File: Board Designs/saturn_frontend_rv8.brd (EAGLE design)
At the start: 38.5 x 30.2 mm, 24 parts

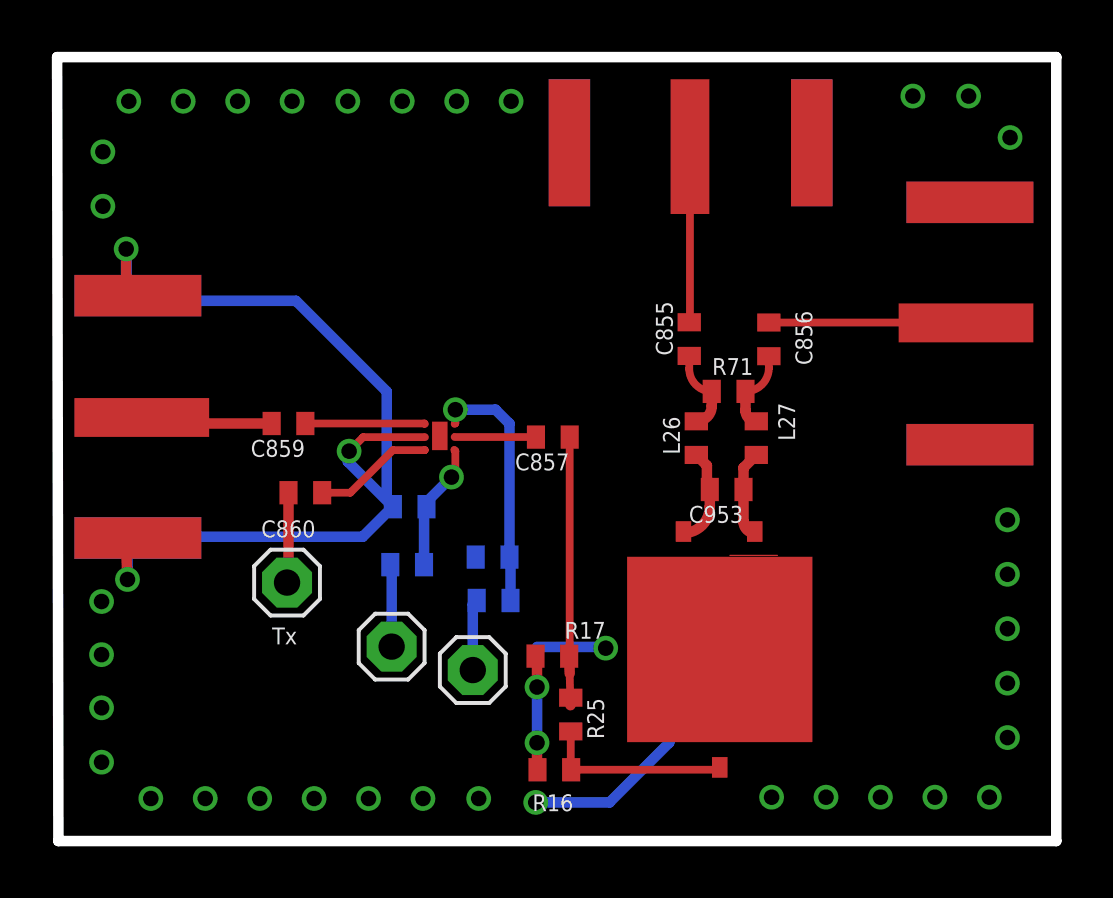
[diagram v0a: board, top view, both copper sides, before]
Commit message: Next Revision of board
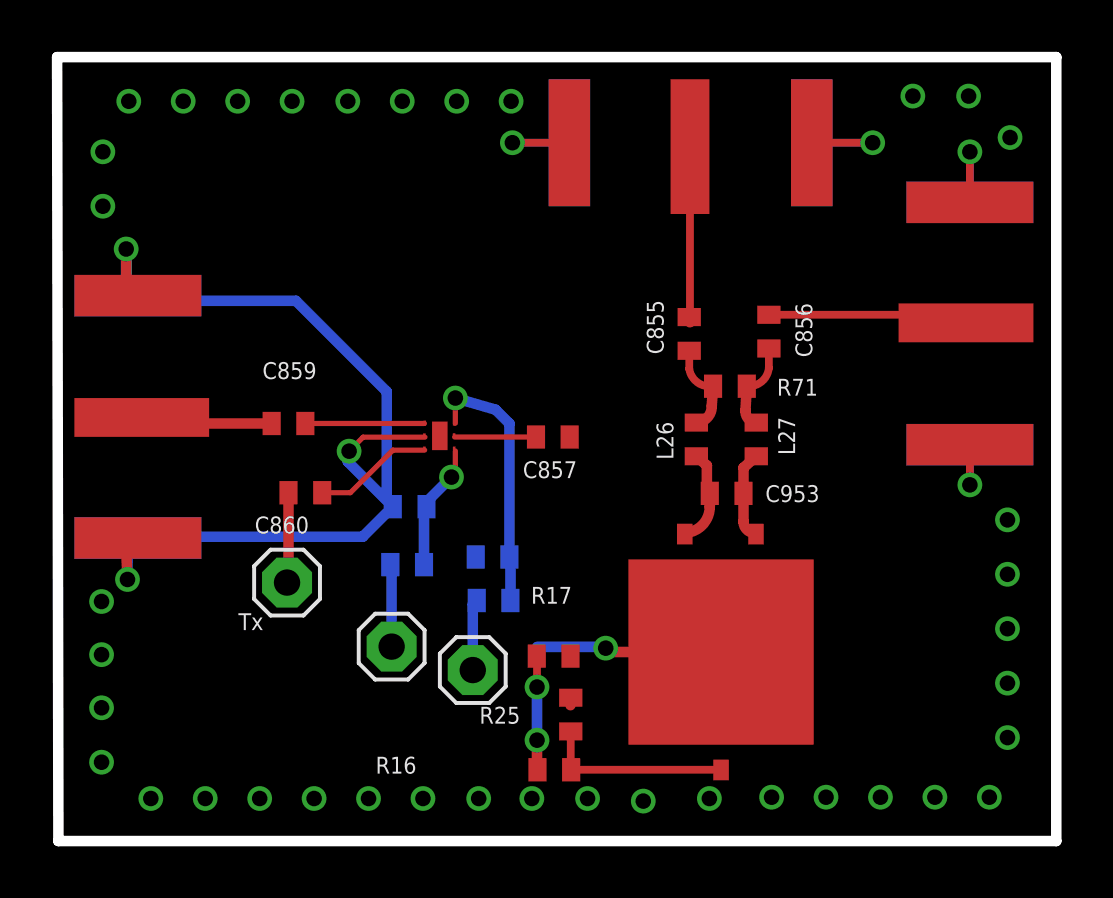
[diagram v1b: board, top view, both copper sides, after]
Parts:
- removed E$1: (no value), cody_custom_library:BALH-0006SMG
- added E$6: (no value), cody_custom_library:BALH-0006SMG
- moved C856 0.30 mm to (39.1, 39.2)
- moved R71 0.21 mm to (37.6, 37.1)
- moved C855 0.20 mm to (36.1, 39.1)
- moved C953 0.15 mm to (37.5, 33.0)
- moved L26 0.05 mm to (36.3, 35.1)
- moved L27 0.05 mm to (38.7, 35.1)
- moved R17 0.05 mm to (30.8, 26.7)
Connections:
- removed net S$8: C857.1, R17.1, R25.1
- new net S$81: R25.1
- net GND: now also E$4.P$1, E$4.P$2, E$5.P$1, E$5.P$2, E$6.GND; no longer E$1.GND
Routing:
- net S$8: track 12.0 -> 0.00 mm, vias 0 -> 1
- net GND: track 59.0 -> 70.3 mm, vias 7 -> 10
- added copper zone on layer 1, net SIGGND
